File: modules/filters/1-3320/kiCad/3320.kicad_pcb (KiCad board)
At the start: 2 copper layers, 40 x 111 mm, 52 parts, among them U2 TL072

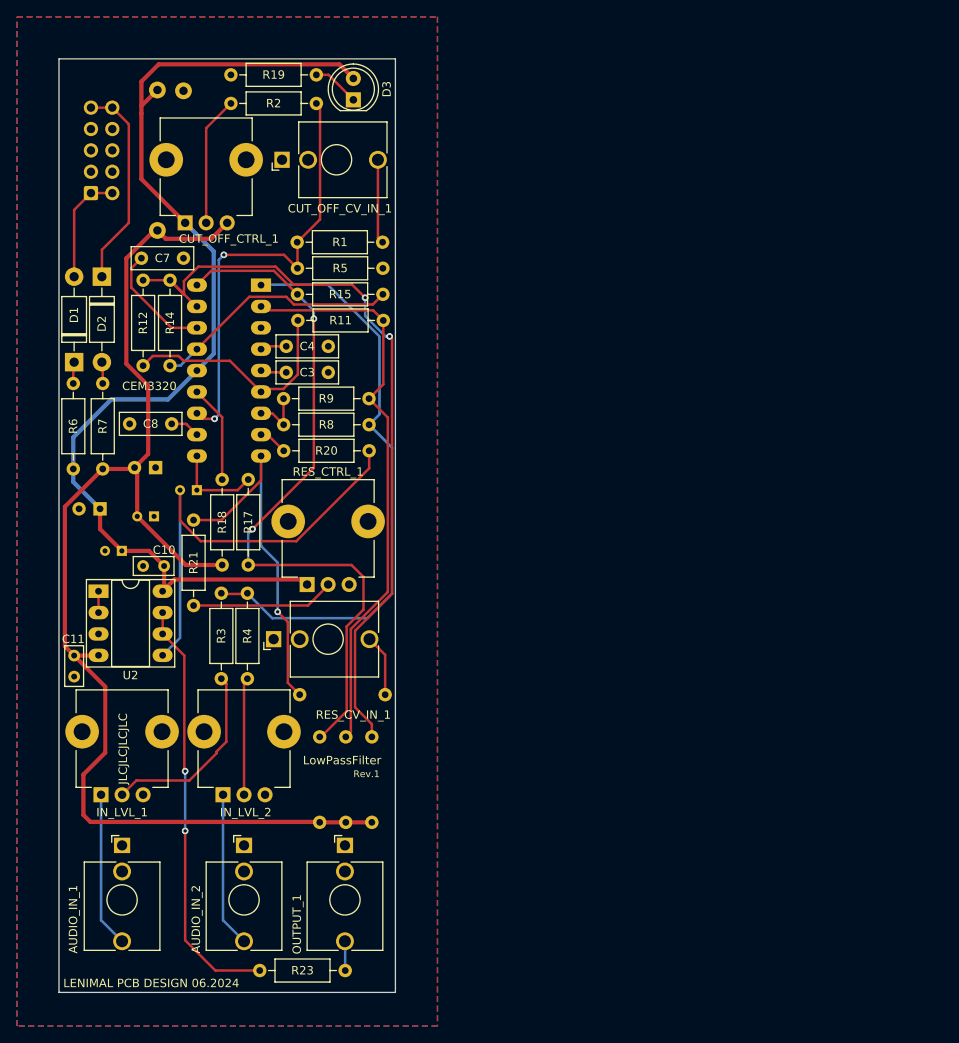
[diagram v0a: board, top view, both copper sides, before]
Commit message: final versions of PCB for modules
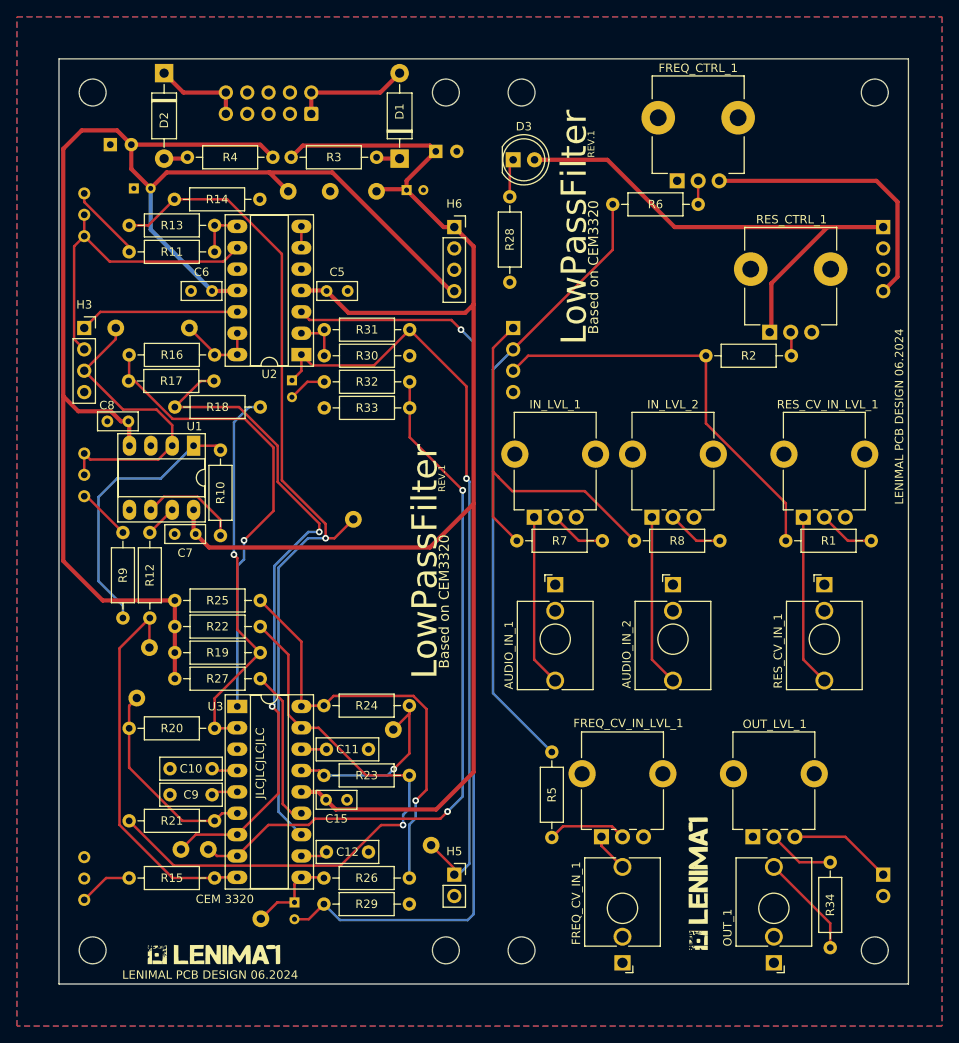
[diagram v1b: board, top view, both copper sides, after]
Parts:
- removed CUT_OFF_CTRL_1: B100K, Synth:Potentiometer_TT_P0915N
- removed CUT_OFF_CV_IN_1: INPUT, Synth:Jack_3.5mm_QingPu_WQP-PJ398SM_Vertical_CircularHoles
- removed OUTPUT_1: OUTPUT, Synth:Jack_3.5mm_QingPu_WQP-PJ398SM_Vertical_CircularHoles
- added C12: 300pF, Synth:C_RECT_WIMA_0.1uF, F.Cu at (86.8, 144.3)
- added C13: 1uF, Capacitor_THT:CP_Radial_D4.0mm_P2.00mm, B.Cu at (78.0, 150.3)
- added C14: 1uF, Capacitor_THT:CP_Radial_D4.0mm_P2.00mm, B.Cu at (77.7, 88.2)
- added C15: 0.1uF, Capacitor_THT:C_Rect_L4.6mm_W2.0mm_P2.50mm_MKS02_FKP02, F.Cu at (84.2, 138.1)
- added FREQ_CTRL_1: B100K, Synth:Potentiometer_TT_P0915N, F.Cu at (126.0, 57.0)
- added FREQ_CV_IN_1: INPUT, Synth:Jack_3.5mm_QingPu_WQP-PJ398SM_Vertical_CircularHoles, F.Cu at (117.0, 151.0)
- added FREQ_CV_IN_LVL_1: B100K, Synth:Potentiometer_Alpha_RD901F-40-00D_Single_Vertical_CircularHoles, F.Cu at (117.0, 135.0)
- added G***: LOGO, Synth:lenimal_logo_full, F.Cu at (68.5, 156.5)
- added G***: LOGO, Synth:lenimal_logo_full, F.Cu at (126.0, 148.0)
- added G***: LOGO, Synth:lenimal_logo_full, B.Cu at (126.0, 148.0)
- added G***: LOGO, Synth:lenimal_logo_full, B.Cu at (68.5, 156.5)
- added H10: MountingHole, MountingHole:MountingHole_3.2mm_M3, F.Cu at (96.0, 54.0)
- added H11: MountingHole, MountingHole:MountingHole_3.2mm_M3, F.Cu at (96.0, 156.0)
- added H12: MountingHole, MountingHole:MountingHole_3.2mm_M3, F.Cu at (105.0, 54.0)
- added H13: MountingHole, MountingHole:MountingHole_3.2mm_M3, F.Cu at (105.0, 156.0)
- added H14: MountingHole, MountingHole:MountingHole_3.2mm_M3, F.Cu at (147.0, 54.0)
- added H15: MountingHole, MountingHole:MountingHole_3.2mm_M3, F.Cu at (147.0, 156.0)
- added H2: PinHeader_01x04, Synth:PinHeader_1x04_P2.54mm_Vertical, B.Cu at (104.0, 82.0)
- added H3: PinSocket_01x04, Synth:PinSocket_1x04_P2.54mm_Vertical, F.Cu at (53.0, 82.0)
- added H4: PinHeader_01x04, Synth:PinHeader_1x04_P2.54mm_Vertical, B.Cu at (148.0, 70.0)
- added H5: PinHeader_01x04, Synth:PinSocket_1x02_P2.54mm_Vertical, F.Cu at (97.0, 147.0)
- added H6: PinSocket_01x04, Synth:PinSocket_1x04_P2.54mm_Vertical, F.Cu at (97.0, 70.0)
- added H7: PinSocket_01x04, Synth:PinHeader_1x02_P2.54mm_Vertical, B.Cu at (148.0, 147.0)
- added H8: MountingHole, MountingHole:MountingHole_3.2mm_M3, F.Cu at (54.0, 54.0)
- added H9: MountingHole, MountingHole:MountingHole_3.2mm_M3, F.Cu at (54.0, 156.0)
- added OUT_1: OUTPUT, Synth:Jack_3.5mm_QingPu_WQP-PJ398SM_Vertical_CircularHoles, F.Cu at (135.0, 151.0)
- added OUT_LVL_1: B100K, Synth:Potentiometer_Alpha_RD901F-40-00D_Single_Vertical_CircularHoles, F.Cu at (135.0, 135.0)
- added R24: 91K, Synth:R_Default (DIN0207), F.Cu at (81.5, 126.9)
- added R25: 220K, Synth:R_Default (DIN0207), F.Cu at (63.8, 114.4)
- added R26: 100K, Synth:R_Default (DIN0207), F.Cu at (81.5, 147.4)
- added R27: 1K8, Synth:R_Default (DIN0207), F.Cu at (73.9, 123.7)
- added R28: 500R, Synth:R_Default (DIN0207), F.Cu at (103.6, 76.5)
- added R29: 68K, Synth:R_Default (DIN0207), F.Cu at (91.6, 150.5)
- added R30: 100K, Synth:R_Default (DIN0207), F.Cu at (91.7, 85.3)
- added R31: 330K, Synth:R_Default (DIN0207), F.Cu at (91.7, 82.2)
- added R32: 51K, Synth:R_Default (DIN0207), F.Cu at (81.6, 88.4)
- added R33: 3K3, Synth:R_Default (DIN0207), F.Cu at (91.7, 91.5)
- added R34: 1K, Synth:R_Default (DIN0207), F.Cu at (141.7, 145.6)
- added RES_CV_IN_LVL_1: B100K, Synth:Potentiometer_Alpha_RD901F-40-00D_Single_Vertical_CircularHoles, F.Cu at (141.0, 97.0)
- added RV1: 50K, Synth:Potentiometer_Bourns_3296W_Vertical, B.Cu at (53.0, 102.0)
- added RV2: 50K, Synth:Potentiometer_Bourns_3296W_Vertical, B.Cu at (53.0, 66.0)
- added RV3: 50K, Synth:Potentiometer_Bourns_3296W_Vertical, B.Cu at (53.0, 150.0)
- added TP10: OUT, Connector_Pin:Pin_D1.0mm_L10.0mm, B.Cu at (94.2, 143.5)
- added TP11: +12V, Connector_Pin:Pin_D1.0mm_L10.0mm, B.Cu at (87.8, 65.8)
- added TP12: GND, Connector_Pin:Pin_D1.0mm_L10.0mm, B.Cu at (82.2, 65.8)
- added TP13: -12V, Connector_Pin:Pin_D1.0mm_L10.0mm, B.Cu at (77.2, 65.8)
- added TP4: RES_CTRL, Connector_Pin:Pin_D1.0mm_L10.0mm, B.Cu at (60.8, 120.0)
- added TP5: POLE_1, Connector_Pin:Pin_D1.0mm_L10.0mm, B.Cu at (64.5, 144.0)
- added TP6: POLE_2, Connector_Pin:Pin_D1.0mm_L10.0mm, B.Cu at (59.2, 126.0)
- added TP7: POLE_3, Connector_Pin:Pin_D1.0mm_L10.0mm, B.Cu at (89.8, 129.8)
- added TP8: POLE_4, Connector_Pin:Pin_D1.0mm_L10.0mm, B.Cu at (74.0, 152.2)
- added TP9: V_RES, Connector_Pin:Pin_D1.0mm_L10.0mm, B.Cu at (67.8, 144.0)
- added U3: ~, Package_DIP:DIP-18_W7.62mm_Socket_LongPads, F.Cu at (71.2, 127.0)
- C10, C11: value 0.1uF -> 300pF; footprint Capacitor_THT:C_Rect_L4.6mm_W2.0mm_P2.50mm_MKS02_FKP02 -> Synth:C_RECT_WIMA_0.1uF
- C3, C4: value 300pF -> 0.1uF; footprint Synth:C_RECT_WIMA_0.1uF -> Capacitor_THT:CP_Radial_D4.0mm_P2.00mm; moved to B.Cu
- C5, C6: footprint Capacitor_THT:CP_Radial_D4.0mm_P2.00mm -> Capacitor_THT:C_Rect_L4.6mm_W2.0mm_P2.50mm_MKS02_FKP02; moved to F.Cu
- C7, C8: value 300pF -> 0.1uF; footprint Synth:C_RECT_WIMA_0.1uF -> Capacitor_THT:C_Rect_L4.6mm_W2.0mm_P2.50mm_MKS02_FKP02
- C9: value 1uF -> 300pF; footprint Capacitor_THT:CP_Radial_D4.0mm_P2.00mm -> Synth:C_RECT_WIMA_0.1uF; moved to F.Cu
- IN_LVL_1, IN_LVL_2: footprint Synth:Potentiometer_TT_P0915N -> Synth:Potentiometer_Alpha_RD901F-40-00D_Single_Vertical_CircularHoles
- R10: value 220K -> 100K; moved to F.Cu
- R11: value 100K -> 68K
- R12: value 91K -> 150K
- R13: value 220K -> 100k; moved to F.Cu
- R14: value 100K -> 1K8
- R15: value 91K -> 1K8
- R16: value 220K -> 91K; moved to F.Cu
- R18: value 1K8 -> 91K
- R19: value 500R -> 220K
- R20: value 51K -> 100K
- R21: value 100K -> 91K
- R22: value 100K -> 220K; moved to F.Cu
- R23: value 1K -> 100K
- R3, R4: value 91K -> 10R
- R5: value 1K8 -> 100K
- R6, R7: value 10R -> 100K
- R9: value 91K -> 68K
- TP1: value +12V -> RES_IN
- TP2: value GND -> F_IN
- TP3: value -12V -> FREQ_CTRL
- U1: value ~ -> TL072; footprint Package_DIP:DIP-18_W7.62mm_Socket_LongPads -> Package_DIP:DIP-8_W7.62mm_Socket_LongPads; moved to F.Cu
- U2: value TL072 -> TL074; footprint Package_DIP:DIP-8_W7.62mm_Socket_LongPads -> Package_DIP:DIP-14_W7.62mm_Socket_LongPads
- moved R13 73.4 mm to (68.5, 69.8), turned to 180 degrees
- moved R15 70.1 mm to (68.5, 147.4), turned to 180 degrees
- moved R19 69.0 mm to (63.8, 120.6)
- moved R1 68.1 mm to (136.4, 107.3)
- moved R6 67.6 mm to (115.9, 67.3), turned to 0 degrees
- moved R5 65.0 mm to (108.6, 132.4), turned to -90 degrees
- moved RES_CTRL_1 62.6 mm to (137.0, 75.0)
- moved IN_LVL_1 61.2 mm to (109.0, 97.0)
- moved IN_LVL_2 60.7 mm to (123.0, 97.0)
- moved AUDIO_IN_1 60.1 mm to (109.0, 119.0)
- moved R16 60.0 mm to (58.4, 85.2), turned to 0 degrees
- moved AUDIO_IN_2 59.7 mm to (123.0, 119.0)
- moved RES_CV_IN_1 59.0 mm to (141.0, 119.0), turned to 0 degrees
- moved C1 58.3 mm to (94.8, 61.0), turned to 0 degrees
- moved R2 55.2 mm to (127.0, 85.3), turned to 0 degrees
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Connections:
- C10 pad 1: +12V -> GNDREF
- C10 pad 2: GNDREF -> Net-(U3-CAP_B)
- C11 pad 2: -12V -> Net-(U3-CAP_C)
- C3 pad 1: GNDREF -> +12V
- C3 pad 2: Net-(U1-CAP_A) -> GNDREF
- C4 pad 2: Net-(U1-CAP_B) -> -12V
- C7 pad 1: GNDREF -> +12V
- C7 pad 2: Net-(U1-CAP_C) -> GNDREF
- C8 pad 2: Net-(U1-CAP_D) -> -12V
- C9 pad 1: Net-(U1-OUT_D) -> GNDREF
- C9 pad 2: Net-(U2B-+) -> Net-(U3-CAP_A)
- R1 pad 1: Net-(U1-FREQ_CTRL) -> Net-(H2C-Pin_3)
- R10 pad 1: -12V -> Net-(U1B--)
- R10 pad 2: Net-(U1-INPUT_B) -> Net-(R10-Pad2)
- R11 pad 1: Net-(U1-OUT_B) -> Net-(R11-Pad1)
- R11 pad 2: Net-(U1-INPUT_B) -> Net-(R11-Pad2)
- R12 pad 1: Net-(U1-INPUT_C) -> Net-(U3-RES_CTRL)
- R12 pad 2: Net-(U1-OUT_B) -> Net-(R12-Pad2)
- R13 pad 1: -12V -> Net-(R11-Pad2)
- R13 pad 2: Net-(U1-INPUT_C) -> Net-(U3-FREQ_CTRL)
- R14 pad 1: Net-(U1-OUT_C) -> Net-(U3-FREQ_CTRL)
- R14 pad 2: Net-(U1-INPUT_C) -> GNDREF
- R15 pad 1: Net-(U1-INPUT_D) -> Net-(U3-RES_CTRL)
- R15 pad 2: Net-(U1-OUT_C) -> Net-(R15-Pad2)
- R16 pad 1: -12V -> Net-(U3-INPUT_A)
- R16 pad 2: Net-(U1-INPUT_D) -> Net-(U2D--)
- R17 pad 1: Net-(U1-OUT_D) -> Net-(U3-OUT_A)
- R17 pad 2: Net-(U1-INPUT_D) -> Net-(U3-INPUT_A)
- R18 pad 1: Net-(U1-IEE) -> Net-(U3-INPUT_B)
- R18 pad 2: -12V -> Net-(U3-OUT_A)
- R19 pad 1: GNDREF -> -12V
- R19 pad 2: Net-(D3-K) -> Net-(U3-INPUT_B)
- R2 pad 1: Net-(U1-FREQ_CTRL) -> Net-(H2C-Pin_3)
- R2 pad 2: Net-(CUT_OFF_CTRL_1-Pad2) -> Net-(R2-Pad2)
- R20 pad 1: Net-(U2B-+) -> Net-(U3-OUT_B)
- R20 pad 2: Net-(U1-FILTER_OUT) -> Net-(U3-INPUT_B)
- R21 pad 1: Net-(U1-RES_CTRL) -> Net-(U3-INPUT_C)
- R21 pad 2: Net-(R21-Pad2) -> Net-(U3-OUT_B)
- R22 pad 1: Net-(U1-RES_CTRL) -> -12V
- R22 pad 2: Net-(R22-Pad2) -> Net-(U3-INPUT_C)
- R23 pad 1: Net-(U2B--) -> Net-(U3-OUT_C)
- R23 pad 2: Net-(OUTPUT_1-PadT) -> Net-(U3-INPUT_C)
- R3 pad 1: Net-(U1-INPUT_A) -> Net-(D1-K)
- R3 pad 2: Net-(IN_LVL_1-Pad2) -> +12V
- R4 pad 1: Net-(U1-INPUT_A) -> Net-(D2-A)
- R4 pad 2: Net-(IN_LVL_2-Pad2) -> -12V
- R5 pad 1: Net-(U1-FREQ_CTRL) -> Net-(H2B-Pin_2)
- R5 pad 2: GNDREF -> Net-(FREQ_CV_IN_LVL_1-Pad2)
- R6 pad 1: Net-(D1-K) -> Net-(H2B-Pin_2)
- R6 pad 2: +12V -> Net-(FREQ_CTRL_1-Pad2)
- R7 pad 1: Net-(D2-A) -> Net-(H2A-Pin_1)
- R7 pad 2: -12V -> Net-(IN_LVL_1-Pad2)
- R8 pad 1: Net-(U1-OUT_A) -> Net-(H2A-Pin_1)
- R8 pad 2: Net-(U1-INPUT_A) -> Net-(IN_LVL_2-Pad2)
- R9 pad 1: Net-(U1-INPUT_B) -> Net-(R9-Pad1)
- R9 pad 2: Net-(U1-OUT_A) -> Net-(R10-Pad2)
- RES_CTRL_1 pad 2: Net-(R21-Pad2) -> Net-(R2-Pad2)
- RES_CV_IN_1 pad T: Net-(R22-Pad2) -> Net-(RES_CV_IN_1-PadT)
- TP1 pad 1: +12V -> Net-(H3C-Pin_3)
- TP2 pad 1: GNDREF -> Net-(U2D--)
- TP3 pad 1: -12V -> Net-(U3-FREQ_CTRL)
- U1 pad 1: Net-(U1-INPUT_A) -> Net-(R10-Pad2)
- U1 pad 2: Net-(U1-INPUT_B) -> Net-(H3C-Pin_3)
- U1 pad 4: Net-(U1-CAP_B) -> -12V
- U1 pad 5: Net-(U1-CAP_A) -> GNDREF
- U1 pad 6: Net-(U1-OUT_B) -> Net-(U1B--)
- U1 pad 7: Net-(U1-OUT_A) -> Net-(R12-Pad2)
- U1 pad 8: Net-(U1-FILTER_OUT) -> +12V
- U2 pad 1: Net-(U2A--) -> Net-(H5A-Pin_1)
- U2 pad 3: GNDREF -> Net-(U2A-+)
- U2 pad 4: -12V -> +12V
- U2 pad 5: Net-(U2B-+) -> GNDREF
- U2 pad 8: +12V -> Net-(R11-Pad2)
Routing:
- net +12V: track 128.9 -> 245.2 mm
- net Net-(U2A-+): track 0.00 -> 113.1 mm, vias 0 -> 1
- net Net-(U3-FREQ_CTRL): track 0.00 -> 102.2 mm, vias 0 -> 1
- net Net-(H5A-Pin_1): track 0.00 -> 92.1 mm, vias 0 -> 1
- net Net-(U1-INPUT_C): track 92.1 -> 0.00 mm, vias 2 -> 0
- net Net-(U1-INPUT_D): track 85.6 -> 0.00 mm, vias 2 -> 0
- net Net-(U3-V_RES): track 0.00 -> 85.4 mm, vias 0 -> 2
- net Net-(U3-OUT_A): track 0.00 -> 81.2 mm, vias 0 -> 2
- net Net-(H2B-Pin_2): track 0.00 -> 73.9 mm
- net Net-(U3-INPUT_C): track 0.00 -> 72.2 mm, vias 0 -> 1
- net Net-(U1-INPUT_A): track 71.6 -> 0.00 mm
- net -12V: track 147.2 -> 216.5 mm
- net Net-(U1-INPUT_B): track 68.5 -> 0.00 mm
- net Net-(U3-INPUT_A): track 0.00 -> 56.2 mm, vias 0 -> 1
- net Net-(U2B-+): track 53.3 -> 0.00 mm
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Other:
- board size 40 x 111 mm -> 101 x 110 mm
- board text added: "AUDIO_IN"
- board text added: "Based on CEM3320"
- board text added: "CEM 3320"
- board text added: "FREQ_CTRL"
- board text added: "OUT"
- board text added: "POLE_1"
- board text added: "POLE_2"
- board text added: "POLE_3"
- board text added: "POLE_4"
- board text added: "RES_CTRL"
- board text added: "RES_IN"
- board text added: "REV.1"
- board text added: "V_RES"
- board text removed: "Based on the CEM 3320"
- board text removed: "CEM3320"
- board text removed: "Low Pass Filter"
- board text removed: "Rev.1"
